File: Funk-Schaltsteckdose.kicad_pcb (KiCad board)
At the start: 2 copper layers, 61 x 96.5 mm, 20 parts, among them J1 L, J2 L', J3 N, K1 G6B-2214P, Q1 BC337, SW1 SW_DIP_x01, U1 ArduinoProMini, U2 LP2950-3.3_TO92, U4 E07_868MS10

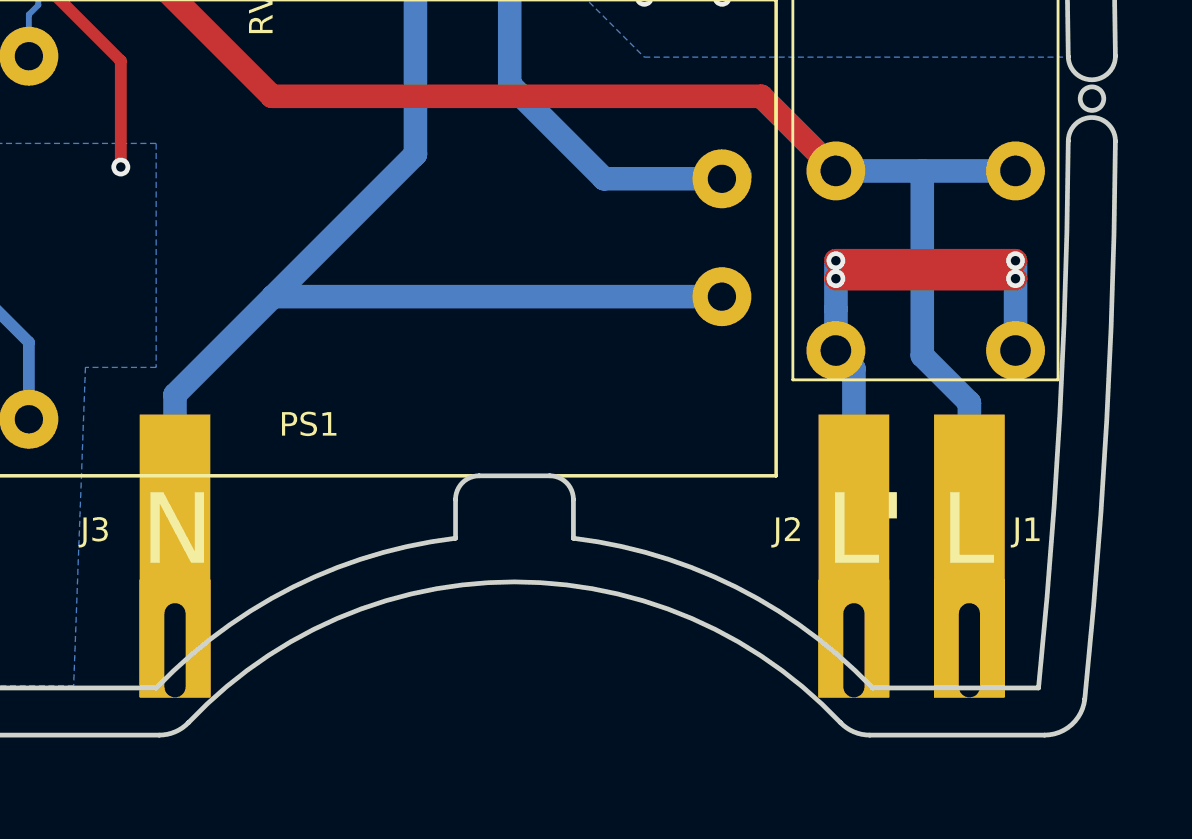
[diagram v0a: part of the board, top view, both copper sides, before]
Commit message: Layout angepasst
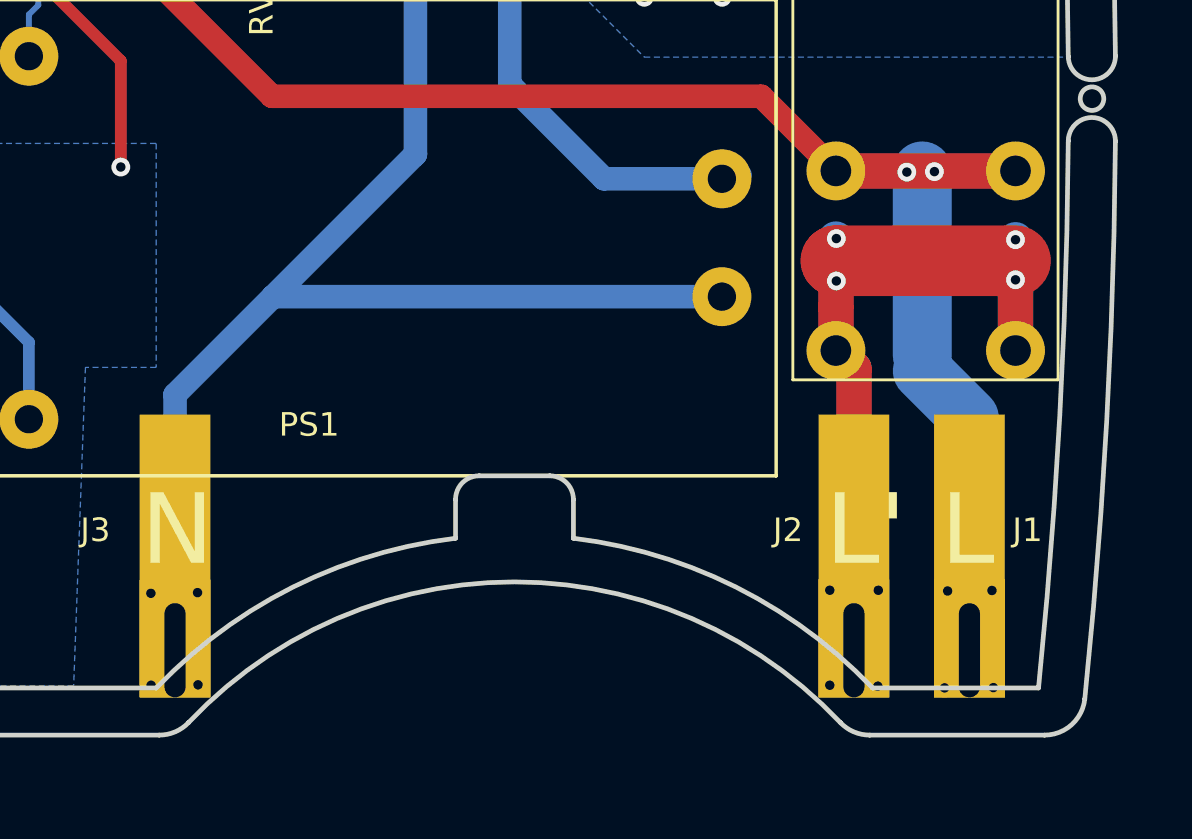
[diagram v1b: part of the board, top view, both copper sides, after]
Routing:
- net Net-(J2-Pad1): track 32.5 -> 44.1 mm, vias 4 -> 8
- net Net-(F1-Pad2): track 60.4 -> 61.6 mm, vias 0 -> 6
- net Net-(J3-Pad1): vias 0 -> 4
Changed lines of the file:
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@@
     (thickness 1.6)
     (drawings 86)
-    (tracks 198)
+    (tracks 221)
     (zones 0)
     (modules 20)
@@
   (gr_line (start 86.03 90.475) (end 86.03 76.505) (layer Edge.Cuts) (width 0.15))
   (gr_line (start 83.49 76.505) (end 83.49 90.475) (layer Edge.Cuts) (width 0.15))
+  (via (at 84.575 148.985) (size 0.8) (drill 0.4) (layers F.Cu B.Cu) (net 8))
+  (via (at 86.555 148.955) (size 0.8) (drill 0.4) (layers F.Cu B.Cu) (net 8))
+  (via (at 86.575 152.865) (size 0.8) (drill 0.4) (layers F.Cu B.Cu) (net 8))
+  (via (at 84.585 152.885) (size 0.8) (drill 0.4) (layers F.Cu B.Cu) (net 8))
+  (via (at 115.435 148.855) (size 0.8) (drill 0.4) (layers F.Cu B.Cu) (net 2))
+  (via (at 115.415 152.925) (size 0.8) (drill 0.4) (layers F.Cu B.Cu) (net 2))
+  (via (at 113.375 152.885) (size 0.8) (drill 0.4) (layers F.Cu B.Cu) (net 2))
+  (via (at 118.245 152.995) (size 0.8) (drill 0.4) (layers F.Cu B.Cu) (net 7))
+  (via (at 120.315 152.985) (size 0.8) (drill 0.4) (layers F.Cu B.Cu) (net 7))
+  (via (at 120.255 148.865) (size 0.8) (drill 0.4) (layers F.Cu B.Cu) (net 7))
+  (via (at 118.375 148.885) (size 0.8) (drill 0.4) (layers F.Cu B.Cu) (net 7))
   (segment (start 109.41 131.4) (end 109.571 131.239) (width 1) (layer B.Cu) (net 1))
   (segment (start 82.8 115.9) (end 86.3 119.4) (width 1) (layer B.Cu) (net 1))
@@
   (segment (start 90.8 119.4) (end 96.3 119.4) (width 1) (layer B.Cu) (net 1))
   (segment (start 96.3 119.4) (end 99.8 122.9) (width 1) (layer B.Cu) (net 1))
-  (segment (start 121.255 138.685) (end 121.255 135.637) (width 1) (layer B.Cu) (net 2))
-  (segment (start 113.635 138.685) (end 114.4 139.45) (width 1) (layer B.Cu) (net 2))
-  (segment (start 114.4 139.45) (end 114.4 148) (width 1) (layer B.Cu) (net 2))
-  (segment (start 113.635 138.685) (end 113.635 136.917234) (width 1) (layer B.Cu) (net 2))
-  (segment (start 113.635 136.917234) (end 113.635 135.637) (width 1) (layer B.Cu) (net 2))
-  (segment (start 113.635 134.875) (end 113.635 134.875) (width 1) (layer B.Cu) (net 2))
-  (via (at 113.635 134.875) (size 0.8) (drill 0.4) (layers F.Cu B.Cu) (net 2))
-  (via (at 121.255 134.875) (size 0.8) (drill 0.4) (layers F.Cu B.Cu) (net 2))
-  (segment (start 113.635 135.637) (end 113.635 134.875) (width 1) (layer B.Cu) (net 2))
-  (via (at 113.635 135.637) (size 0.8) (drill 0.4) (layers F.Cu B.Cu) (net 2))
-  (segment (start 121.255 135.637) (end 121.255 134.875) (width 1) (layer B.Cu) (net 2))
-  (via (at 121.255 135.637) (size 0.8) (drill 0.4) (layers F.Cu B.Cu) (net 2))
-  (segment (start 113.635 134.875) (end 121.255 134.875) (width 1) (layer F.Cu) (net 2))
-  (segment (start 113.635 135.637) (end 121.255 135.637) (width 1) (layer F.Cu) (net 2))
+  (segment (start 113.635 138.685) (end 114.4 139.45) (width 1.5) (layer B.Cu) (net 2))
+  (segment (start 114.4 139.45) (end 114.4 148) (width 1.5) (layer B.Cu) (net 2))
+  (segment (start 113.635 134.875) (end 113.655 134.875) (width 3) (layer F.Cu) (net 2))
+  (segment (start 113.635 138.685) (end 113.635 136.835) (width 1.5) (layer F.Cu) (net 2))
+  (segment (start 121.255 138.685) (end 121.255 136.135) (width 1.5) (layer F.Cu) (net 2))
+  (via (at 113.375 148.855) (size 0.8) (drill 0.4) (layers F.Cu B.Cu) (net 2))
+  (segment (start 113.635 138.685) (end 113.635 138.715) (width 1) (layer F.Cu) (net 2))
+  (segment (start 113.635 138.715) (end 114.405 139.485) (width 1.5) (layer F.Cu) (net 2))
+  (segment (start 113.655 134.875) (end 121.255 134.875) (width 3) (layer F.Cu) (net 2))
+  (via (at 113.655 133.935) (size 0.8) (drill 0.4) (layers F.Cu B.Cu) (net 2))
+  (segment (start 121.255 134.885) (end 121.255 134.875) (width 1.5) (layer F.Cu) (net 2))
+  (via (at 121.255 133.985) (size 0.8) (drill 0.4) (layers F.Cu B.Cu) (net 2))
+  (segment (start 121.255 136.135) (end 121.255 134.885) (width 1.5) (layer F.Cu) (net 2))
+  (via (at 121.255 135.685) (size 0.8) (drill 0.4) (layers F.Cu B.Cu) (net 2))
+  (segment (start 113.655 134.875) (end 113.655 134.875) (width 3) (layer F.Cu) (net 2))
+  (via (at 113.655 135.735) (size 0.8) (drill 0.4) (layers F.Cu B.Cu) (net 2))
+  (segment (start 113.635 136.835) (end 113.635 134.875) (width 1.5) (layer F.Cu) (net 2))
+  (segment (start 113.635 133.955) (end 113.655 133.935) (width 1) (layer B.Cu) (net 2))
+  (segment (start 113.635 138.685) (end 113.635 133.955) (width 1.5) (layer B.Cu) (net 2))
+  (segment (start 121.255 138.685) (end 121.255 133.985) (width 1.5) (layer B.Cu) (net 2))
+  (segment (start 114.4 139.45) (end 114.4 148.15) (width 1.5) (layer F.Cu) (net 2))
   (segment (start 105.08 92.38) (end 106.35 93.65) (width 0.25) (layer B.Cu) (net 3))
   (segment (start 105.08 91.279029) (end 105.08 92.38) (width 0.25) (layer B.Cu) (net 3))
@@
   (segment (start 82.79 120.98) (end 89.71 127.9) (width 1) (layer F.Cu) (net 7))
   (segment (start 89.71 127.9) (end 110.47 127.9) (width 1) (layer F.Cu) (net 7))
-  (segment (start 117.3 131.065) (end 117.3 138.9) (width 1) (layer B.Cu) (net 7))
-  (segment (start 117.3 131.065) (end 121.255 131.065) (width 1) (layer B.Cu) (net 7))
-  (segment (start 113.635 131.065) (end 117.3 131.065) (width 1) (layer B.Cu) (net 7))
-  (segment (start 119.3 140.9) (end 119.3 148) (width 1) (layer B.Cu) (net 7))
-  (segment (start 117.3 138.9) (end 119.3 140.9) (width 1) (layer B.Cu) (net 7))
+  (segment (start 117.3 131.065) (end 117.3 131.065) (width 2.5) (layer B.Cu) (net 7))
+  (segment (start 117.3 131.065) (end 121.255 131.065) (width 1.5) (layer B.Cu) (net 7))
+  (segment (start 113.635 131.065) (end 117.3 131.065) (width 1.5) (layer B.Cu) (net 7))
+  (segment (start 113.635 131.065) (end 121.255 131.065) (width 1.5) (layer F.Cu) (net 7))
+  (segment (start 117.3 131.065) (end 117.3 138.9) (width 2.5) (layer B.Cu) (net 7))
+  (via (at 116.645 131.115) (size 0.8) (drill 0.4) (layers F.Cu B.Cu) (net 7))
+  (segment (start 117.3 131.065) (end 117.3 131.065) (width 2.5) (layer B.Cu) (net 7))
+  (via (at 117.815 131.095) (size 0.8) (drill 0.4) (layers F.Cu B.Cu) (net 7))
+  (segment (start 117.3 139.55) (end 117.3 138.9) (width 1) (layer B.Cu) (net 7))
+  (segment (start 119.3 141.55) (end 117.3 139.55) (width 2.5) (layer B.Cu) (net 7))
   (segment (start 85.6 140.558) (end 85.6 148) (width 1) (layer B.Cu) (net 8))
   (segment (start 108.8 136.4) (end 89.758 136.4) (width 1) (layer B.Cu) (net 8))
